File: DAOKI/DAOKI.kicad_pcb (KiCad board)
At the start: 2 copper layers, 14 parts, among them CON4 CON4, U1 MOCH22a1, U2 LM393

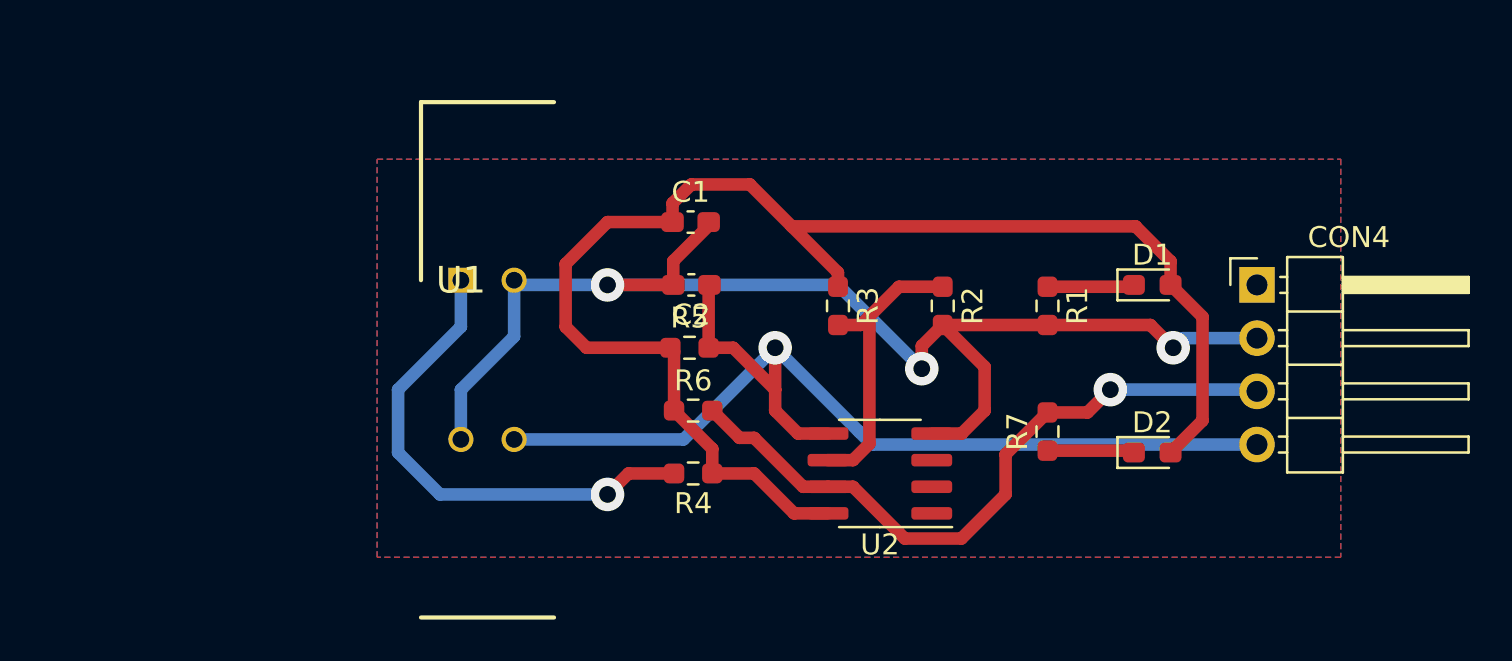
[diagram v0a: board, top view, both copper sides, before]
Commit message: New routing
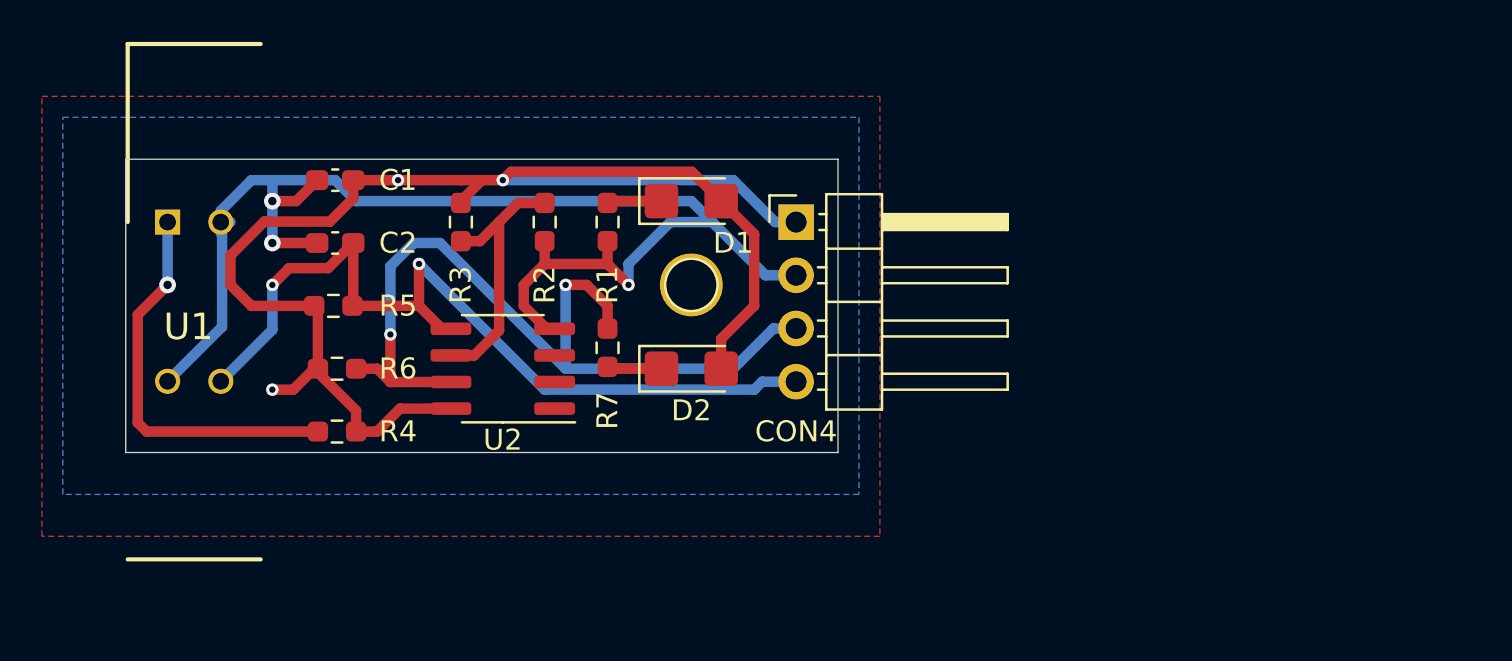
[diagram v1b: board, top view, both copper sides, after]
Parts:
- added REF**: Pin_D1.0mm_L10.0mm, Connector_Pin:Pin_D1.0mm_L10.0mm, F.Cu at (150.0, 94.0)
- D1, D2: footprint LED_SMD:LED_0603_1608Metric_Pad1.05x0.95mm_HandSolder -> LED_SMD:LED_1206_3216Metric_Castellated
- moved D1 22.4 mm to (150.0, 90.0)
- moved D2 22.4 mm to (150.0, 98.0)
- moved CON4 22.2 mm to (155.0, 91.0)
- moved R1 21.4 mm to (146.0, 91.0)
- moved R7 21.4 mm to (146.0, 97.0)
- moved R2 19.4 mm to (143.0, 91.0)
- moved U2 18.7 mm to (141.0, 98.0)
- moved R3 18.4 mm to (139.0, 91.0)
- moved C2 17.1 mm to (133.0, 92.0)
- moved R4 17.1 mm to (133.1, 101.0)
- moved R5 17.1 mm to (132.9, 95.0)
- moved R6 17.1 mm to (133.1, 98.0)
- moved C1 17.1 mm to (133.0, 89.0), turned to 180 degrees
- moved U1 14.3 mm to (125.0, 91.0)
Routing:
- net Net-(C2-Pad1): track 52.2 -> 40.6 mm, vias 1 -> 2
- net Net-(CON4-Pad3): track 32.6 -> 40.9 mm, vias 1 -> 2
- net Net-(R4-Pad2): track 23.9 -> 19.1 mm
- net +5V: track 68.2 -> 72.0 mm, vias 0 -> 3
- net GND: track 62.7 -> 64.6 mm
- net Net-(D2-Pad1): track 4.16 -> 2.61 mm
- net Net-(D1-Pad1): track 4.16 -> 2.61 mm
- net Net-(R2-Pad1): track 14.1 -> 12.7 mm
- added copper zone on B.Cu, net +5V
- added copper zone on F.Cu, net GND
- removed copper zone on F.Cu, net +5V
- removed copper zone on B.Cu, net GND
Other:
- board outline added: 34 x 14 mm
